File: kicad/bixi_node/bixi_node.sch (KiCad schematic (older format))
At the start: 8 parts, among them J1 RJ45, J2 Screw_Terminal_1x01, J3 Screw_Terminal_1x01, P1 CONN_01X03, U1 SP3485CN

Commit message: v2 pcb
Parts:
- C1: footprint Resistors_THT:Resistor_Horizontal_RM7mm -> Capacitors_THT:C_Disc_D3.0mm_W2.0mm_P2.50mm
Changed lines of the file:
@@
 F 0 "C1" H 4375 4950 50  0000 L CNN
 F 1 "C" H 4375 4750 50  0000 L CNN
-F 2 "Resistors_THT:Resistor_Horizontal_RM7mm" H 4388 4700 50  0001 C CNN
+F 2 "Capacitors_THT:C_Disc_D3.0mm_W2.0mm_P2.50mm" H 4388 4700 50  0001 C CNN
 F 3 "" H 4350 4850 50  0000 C CNN
 	1    4350 4850

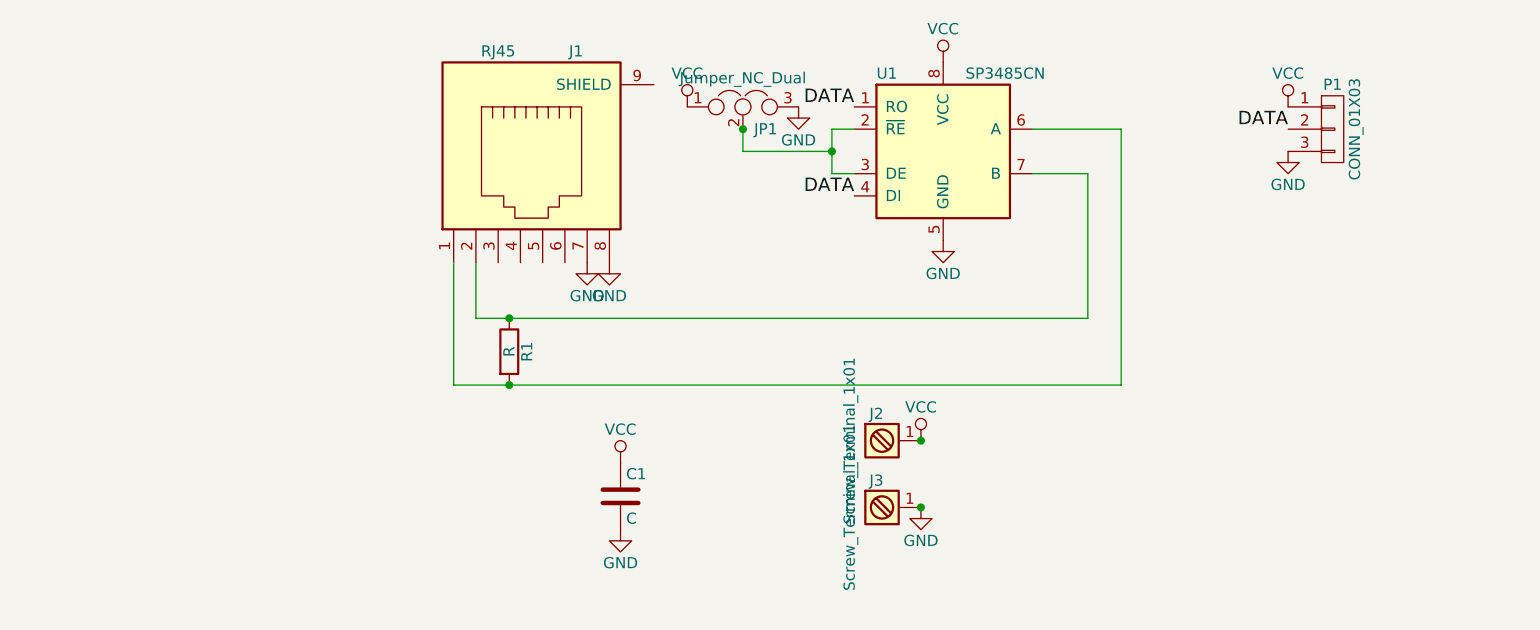
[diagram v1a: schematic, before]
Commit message: bixi node updates
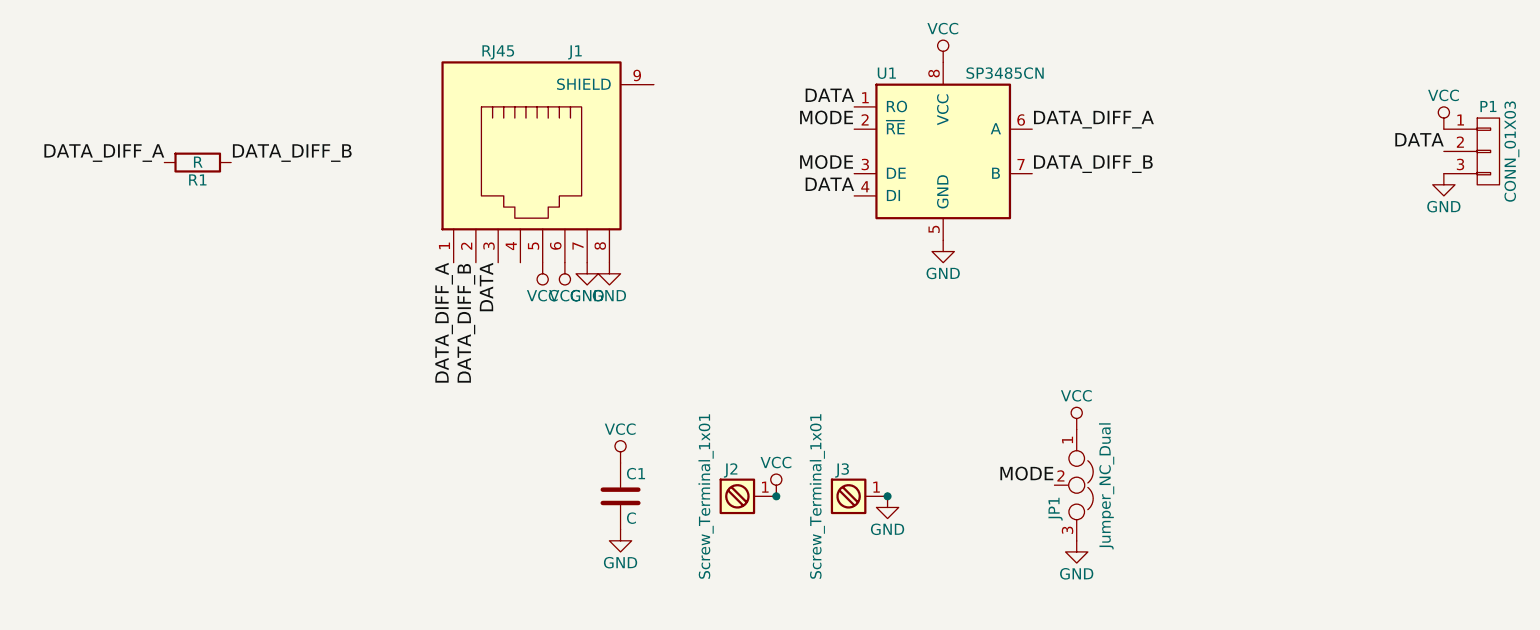
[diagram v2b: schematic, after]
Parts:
- C1: footprint Capacitors_THT:C_Disc_D3.0mm_W2.0mm_P2.50mm -> Capacitors_THT:C_Axial_L3.8mm_D2.6mm_P7.50mm_Horizontal
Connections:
- net DATA: now also J1.3
- net VCC: now also J1.5, J1.6
- net DATA_DIFF_A: now reaches J1.1, R1.2, U1.6 (A)
- net DATA_DIFF_B: now reaches J1.2, R1.1, U1.7 (B)
- net MODE: now reaches JP1.2, U1.2 (~RE~), U1.3 (DE)
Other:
- moved on the sheet: J2, J3, JP1, P1
